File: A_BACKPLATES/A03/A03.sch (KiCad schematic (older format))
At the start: 74 parts, among them J0 Conn_01x01_Male, J1 Conn_01x01_Male, J2 Conn_01x01_Male, J3 Conn_01x01_Male

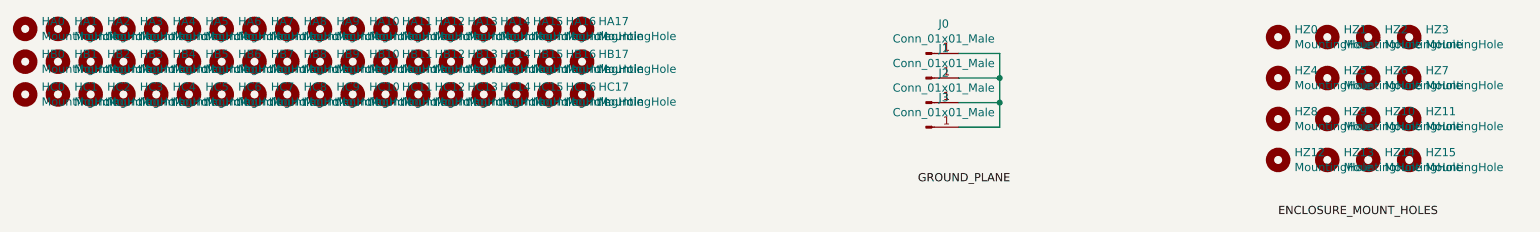
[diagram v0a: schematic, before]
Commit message: A03 finished
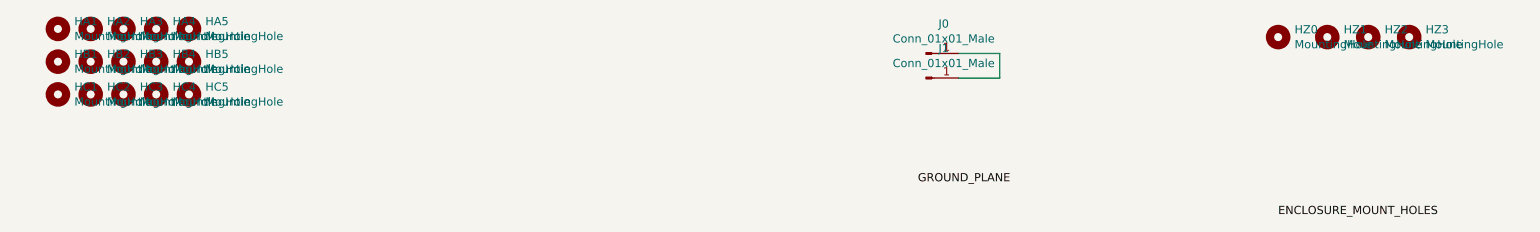
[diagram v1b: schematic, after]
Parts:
- removed HA0, HA10, HA11, HA12, HA13, HA14, HA15, HA16, HA17, HA6, HA7, HA8, HA9, HB0, HB10, HB11, HB12, HB13, HB14, HB15, HB16, HB17, HB6, HB7, HB8, HB9, HC0, HC10, HC11, HC12, HC13, HC14, HC15, HC16, HC17, HC6, HC7, HC8, HC9, HZ10, HZ11, HZ12, HZ13, HZ14, HZ15, HZ4, HZ5, HZ6, HZ7, HZ8, HZ9: MountingHole, MountingHole:MountingHole_3mm, symbol Mechanical:MountingHole
- removed J2, J3: Conn_01x01_Male, Connector_Wire:SolderWirePad_1x01_Drill1mm, symbol Connector:Conn_01x01_Male
